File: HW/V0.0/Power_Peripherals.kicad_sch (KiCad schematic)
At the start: 54 parts, among them Q10 TVS_2CH, Q3 <name>, Q4 <name>, Q5 <name>, Q6 <name>, Q7 <name>, U1 3.3V/300mA, U5 28V/3A Bck

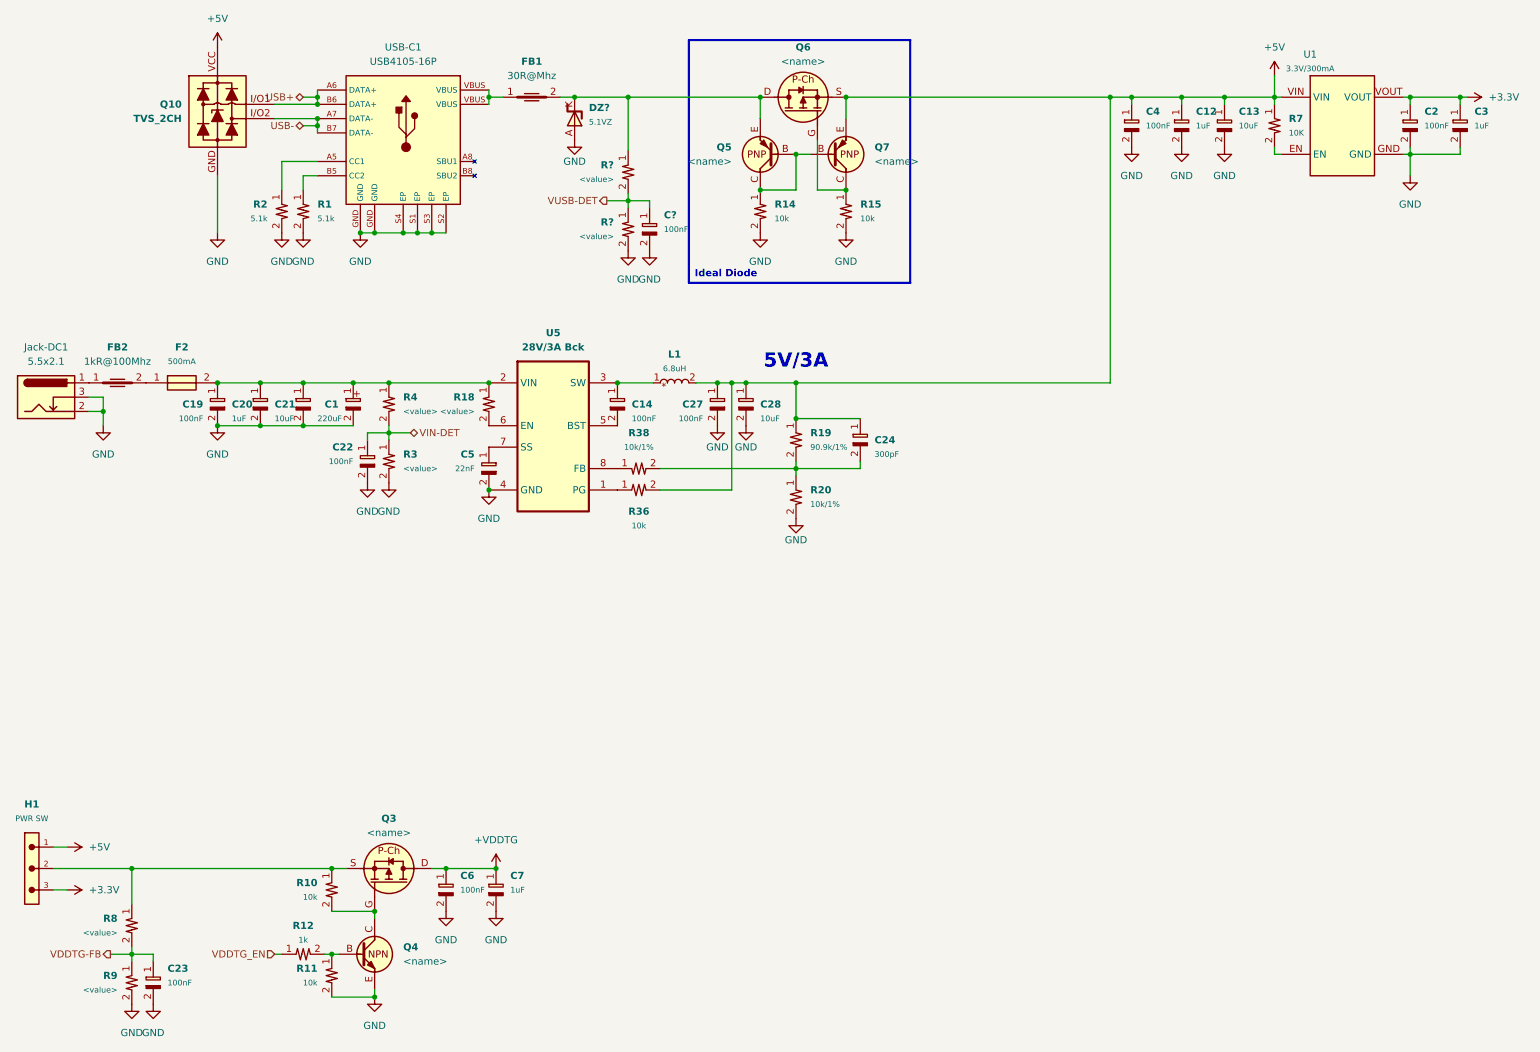
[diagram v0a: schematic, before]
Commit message: PIC16-DevKit-SCH-877 schematic update 1
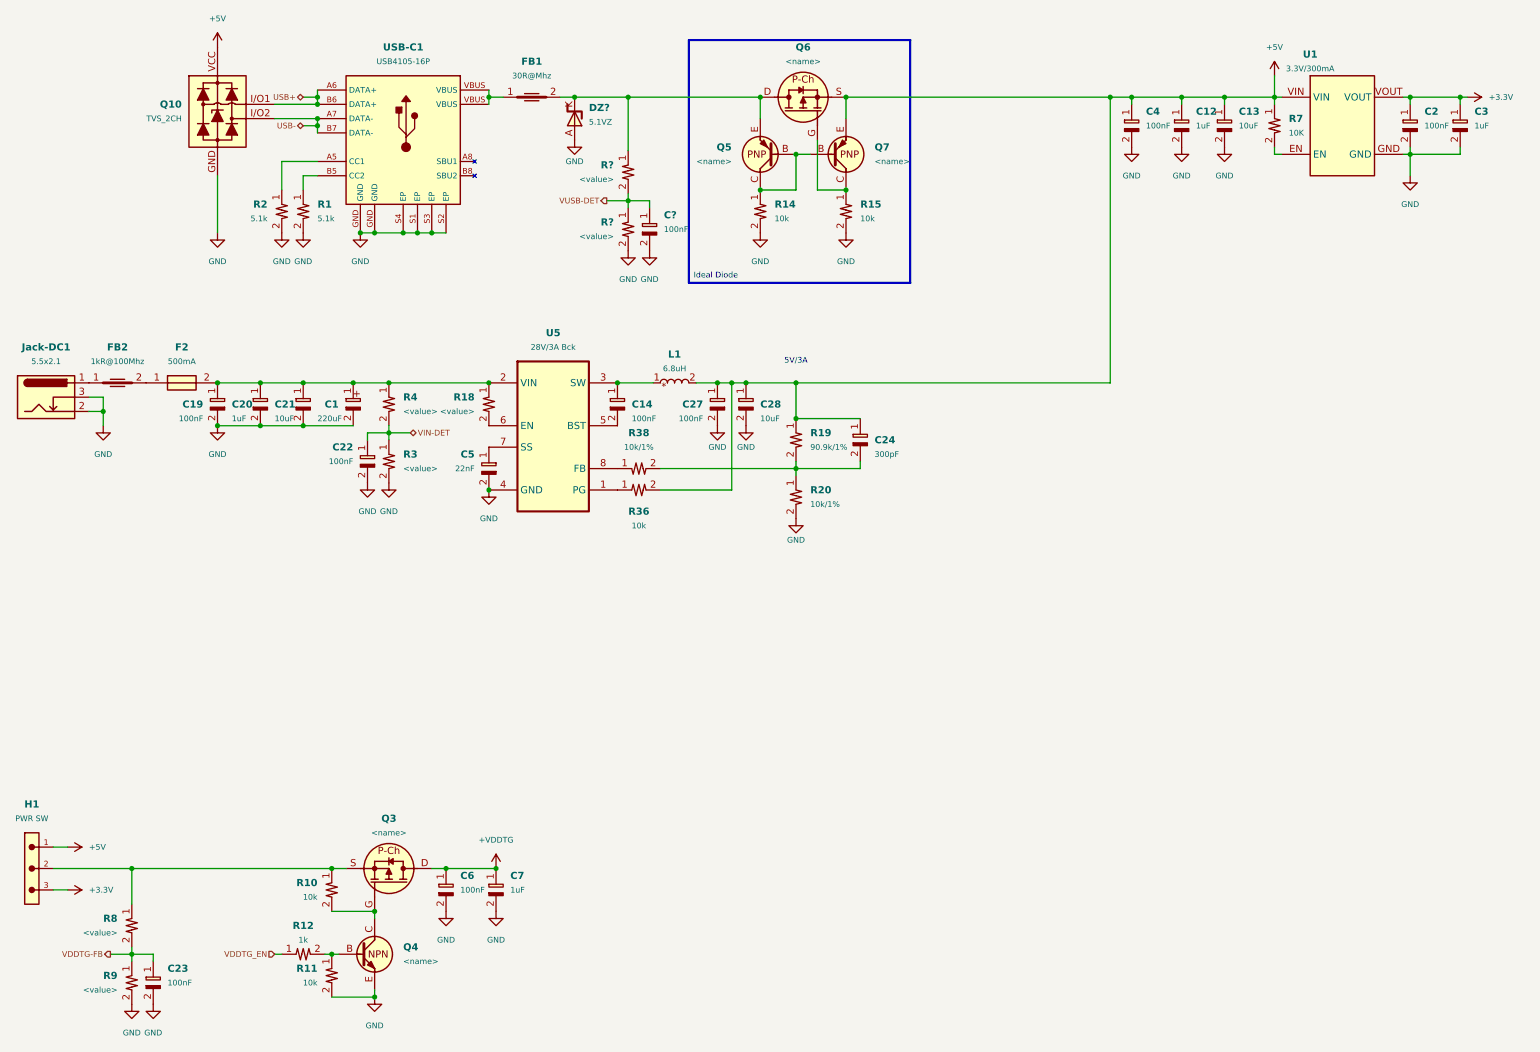
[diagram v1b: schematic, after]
